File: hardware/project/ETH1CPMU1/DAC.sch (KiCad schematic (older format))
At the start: 26 parts, among them U1101 REF192, U1102 TL072, U1103 AD5689BRUZ

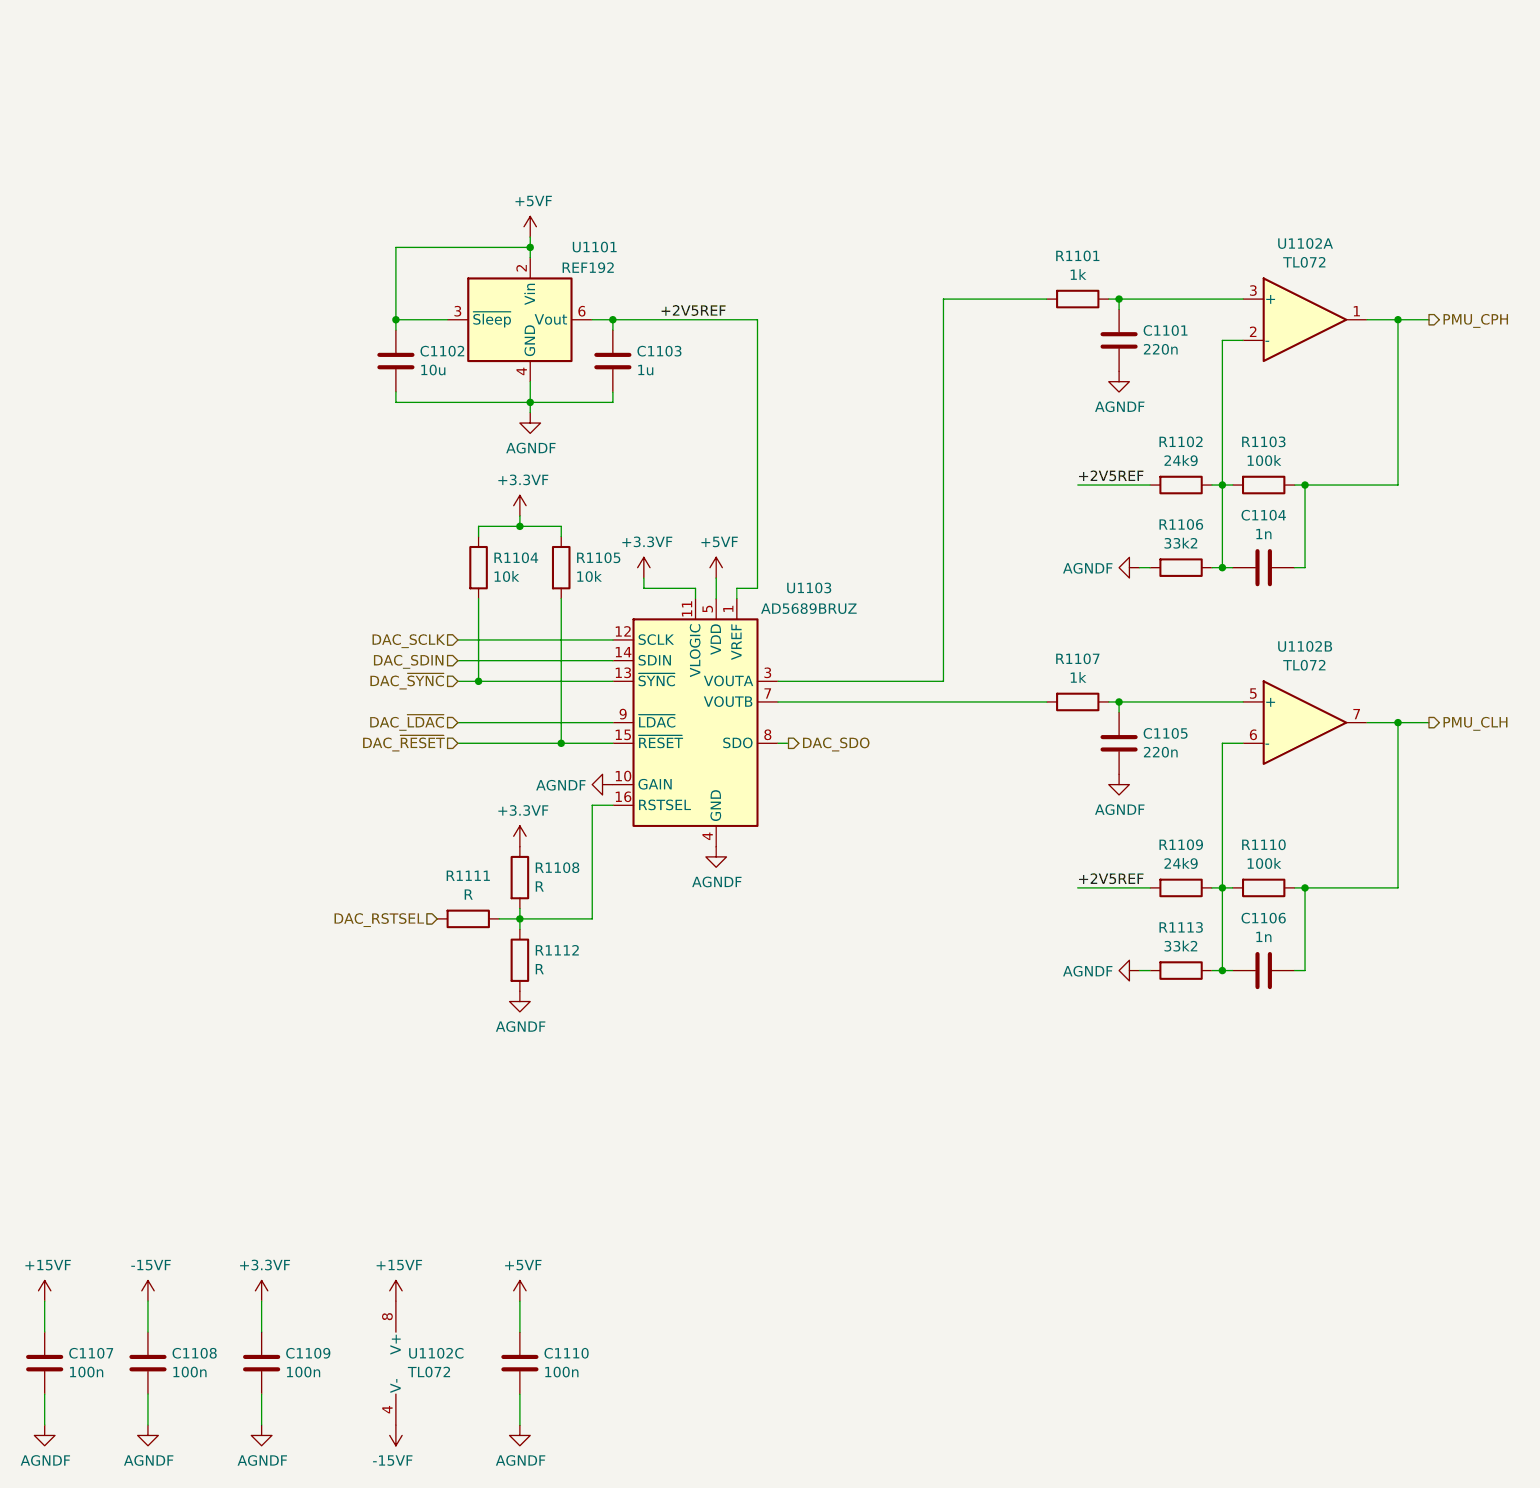
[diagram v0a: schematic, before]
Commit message: PCB design
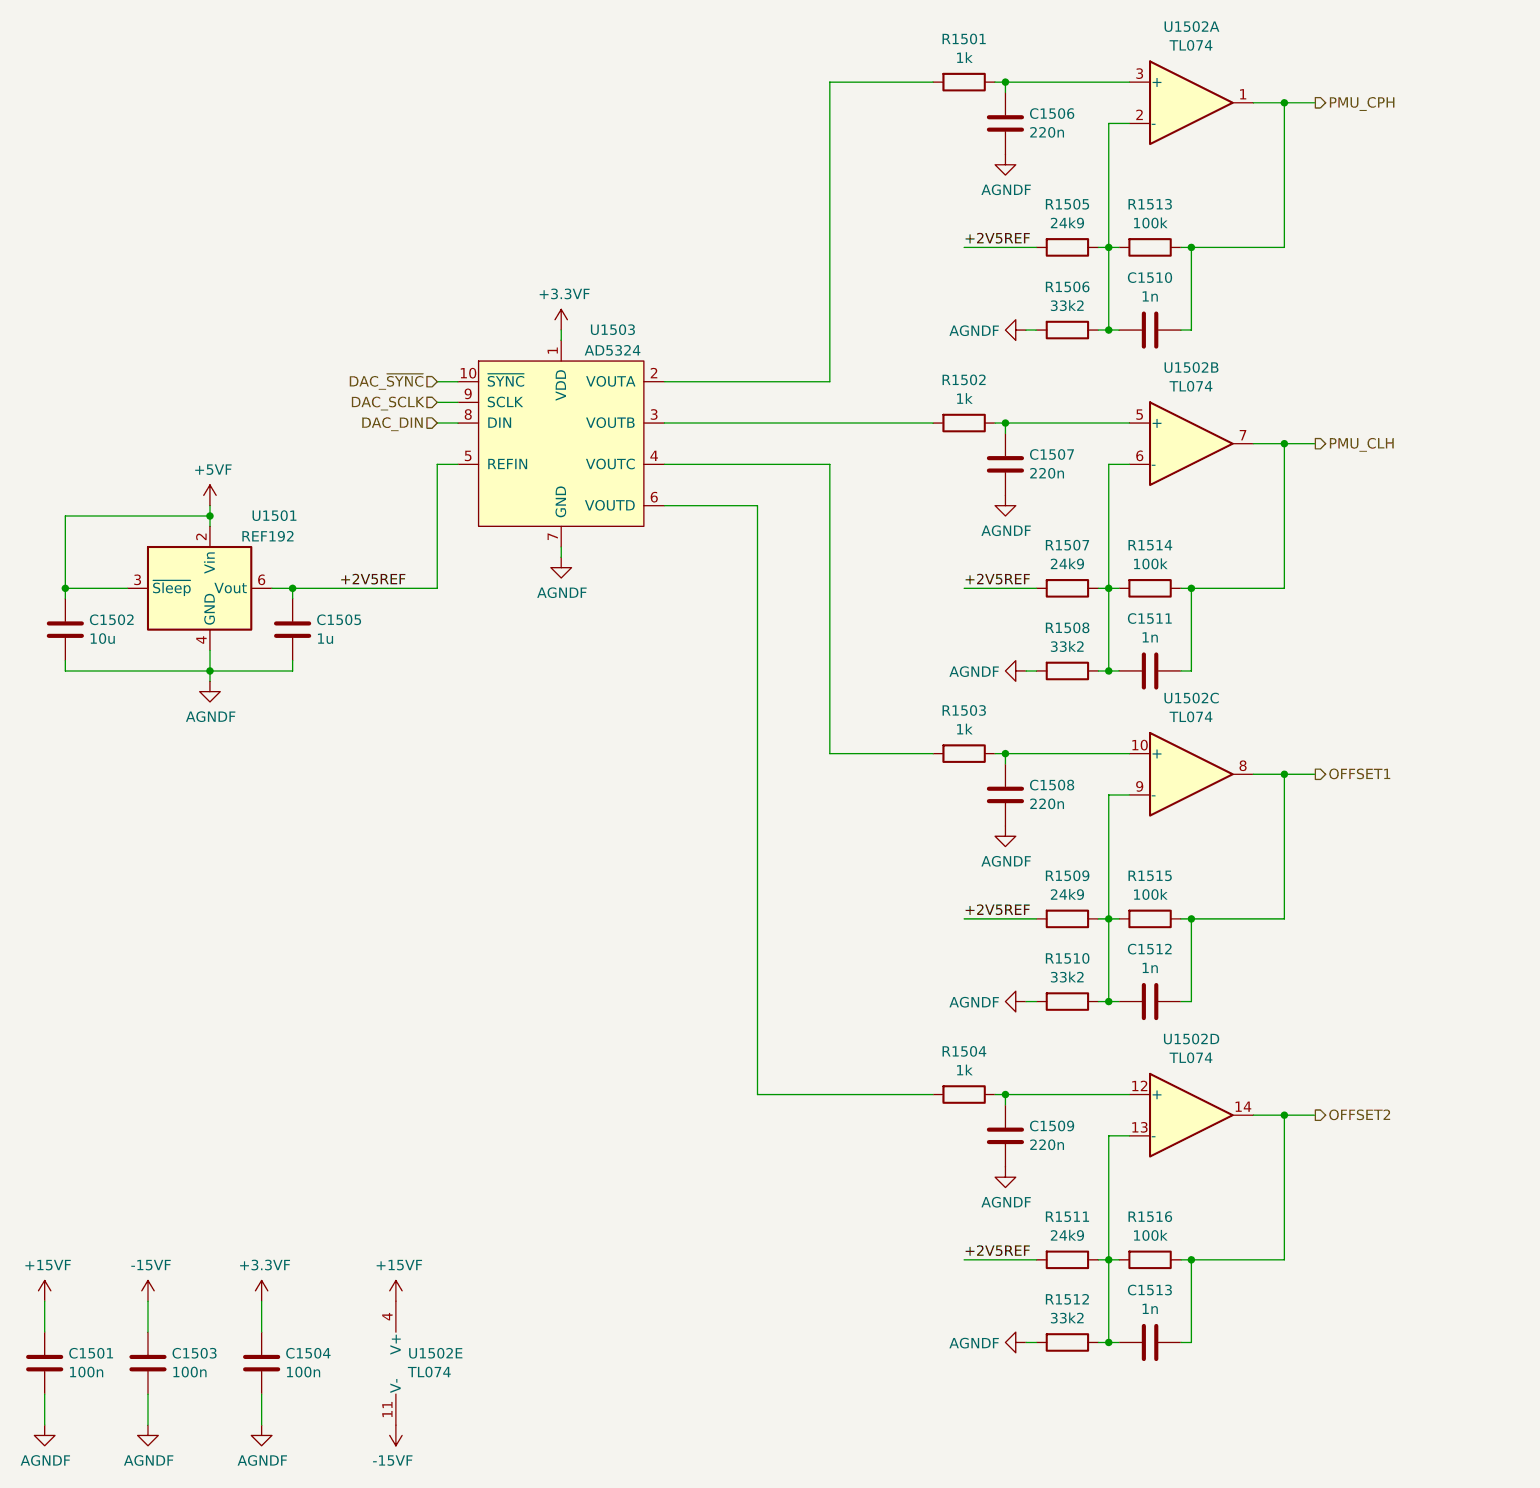
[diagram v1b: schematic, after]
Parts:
- removed C1110: 100n, Capacitor_SMD:C_0603_1608Metric_Pad1.05x0.95mm_HandSolder, symbol Device:C
- removed R1104, R1105: 10k, Resistor_SMD:R_0603_1608Metric_Pad1.05x0.95mm_HandSolder, symbol Device:R
- removed R1108, R1111, R1112: R, Resistor_SMD:R_0603_1608Metric_Pad1.05x0.95mm_HandSolder, symbol Device:R
- removed U1102: TL072, Package_SO:SOIC-8_3.9x4.9mm_P1.27mm, symbol Amplifier_Operational:TL072
- removed U1103: AD5689BRUZ, Package_SO:TSSOP-16_4.4x5mm_P0.65mm, symbol Analog_DAC:AD5689BRUZ
- added C1508, C1509: 220n, Capacitor_SMD:C_0603_1608Metric_Pad1.05x0.95mm_HandSolder, symbol Device:C
- added C1512, C1513: 1n, Capacitor_SMD:C_0603_1608Metric_Pad1.05x0.95mm_HandSolder, symbol Device:C
- added R1503, R1504: 1k, Resistor_SMD:R_0603_1608Metric_Pad1.05x0.95mm_HandSolder, symbol Device:R
- added R1509, R1511: 24k9, Resistor_SMD:R_0603_1608Metric_Pad1.05x0.95mm_HandSolder, symbol Device:R
- added R1510, R1512: 33k2, Resistor_SMD:R_0603_1608Metric_Pad1.05x0.95mm_HandSolder, symbol Device:R
- added R1515, R1516: 100k, Resistor_SMD:R_0603_1608Metric_Pad1.05x0.95mm_HandSolder, symbol Device:R
- added U1502: TL074, Package_SO:SOIC-14_3.9x8.7mm_P1.27mm, symbol Amplifier_Operational:TL074
- added U1503: AD5324, Package_SO:MSOP-10_3x3mm_P0.5mm, symbol ETH1CPMU1:AD5324
- renumbered C1107 to C1501, C1102 to C1502, C1108 to C1503, C1109 to C1504, C1103 to C1505, C1101 to C1506, C1105 to C1507, C1104 to C1510, C1106 to C1511, R1101 to R1501, R1107 to R1502, R1102 to R1505, R1106 to R1506, R1109 to R1507, R1113 to R1508, R1103 to R1513, R1110 to R1514, U1101 to U1501
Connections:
- net +15VF: now also U1502.4 (V+)
- net +2V5REF: now also R1509.2, R1511.2, U1503.5 (REFIN)
- net +3.3VF: now also U1503.1 (VDD)
- net -15VF: now also U1502.11 (V-)
- net AGNDF: now also C1508.2, C1509.2, R1510.2, R1512.2, U1503.7 (GND)
- net DAC_SCLK: now also U1503.9 (SCLK)
- net DAC_~SYNC: now also U1503.10 (~SYNC)
- net PMU_CLH: now also U1502.7
- net PMU_CPH: now also U1502.1
- net at R1501.2: now also U1503.2 (VOUTA)
- net at R1502.2: now also U1503.3 (VOUTB)
- net at C1511.2, R1507.1, R1508.1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: now also U1502.6 (-)
- net at C1507.1, R1502.1: now also U1502.5 (+)
- net at C1510.2, R1505.1, R1506.1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: now also U1502.2 (-)
- net at C1506.1, R1501.1: now also U1502.3 (+)
- new net: R1503.2, U1503.4 (VOUTC)
- new net: R1504.2, U1503.6 (VOUTD)
- new net: C1508.1, R1503.1, U1502.10 (+)
- new net: C1512.2, R1509.1, R1510.1, R1515.2, U1502.9 (-)
- new net: C1509.1, R1504.1, U1502.12 (+)
- new net: C1513.2, R1511.1, R1512.1, R1516.2, U1502.13 (-)
- new net DAC_DIN: U1503.8 (DIN)
- new net OFFSET1: C1512.1, R1515.1, U1502.8
- new net OFFSET2: C1513.1, R1516.1, U1502.14
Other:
- moved on the sheet: C1502, C1505, C1506, C1507, C1510, C1511, R1501, R1502, R1505, R1506, R1507, R1508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
